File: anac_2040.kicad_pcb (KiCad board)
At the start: 2 copper layers, 53.2 x 68.2 mm, 62 parts, among them J1 Conn_01x02, J10 Debug, J5 Conn_01x09, J6 Barrel_Jack_MountingPin, J7 USB_C_Receptacle_USB2.0, Q1 PJA3432AU, Q2 PJA3432AU, SW1 SW_Push, SW2 SW_Push, U1 RP2040, U2 W25Q16JVSSIQ, U3 LM4040DBZ-3, U4 AP63203WU, Y1 Crystal_Small

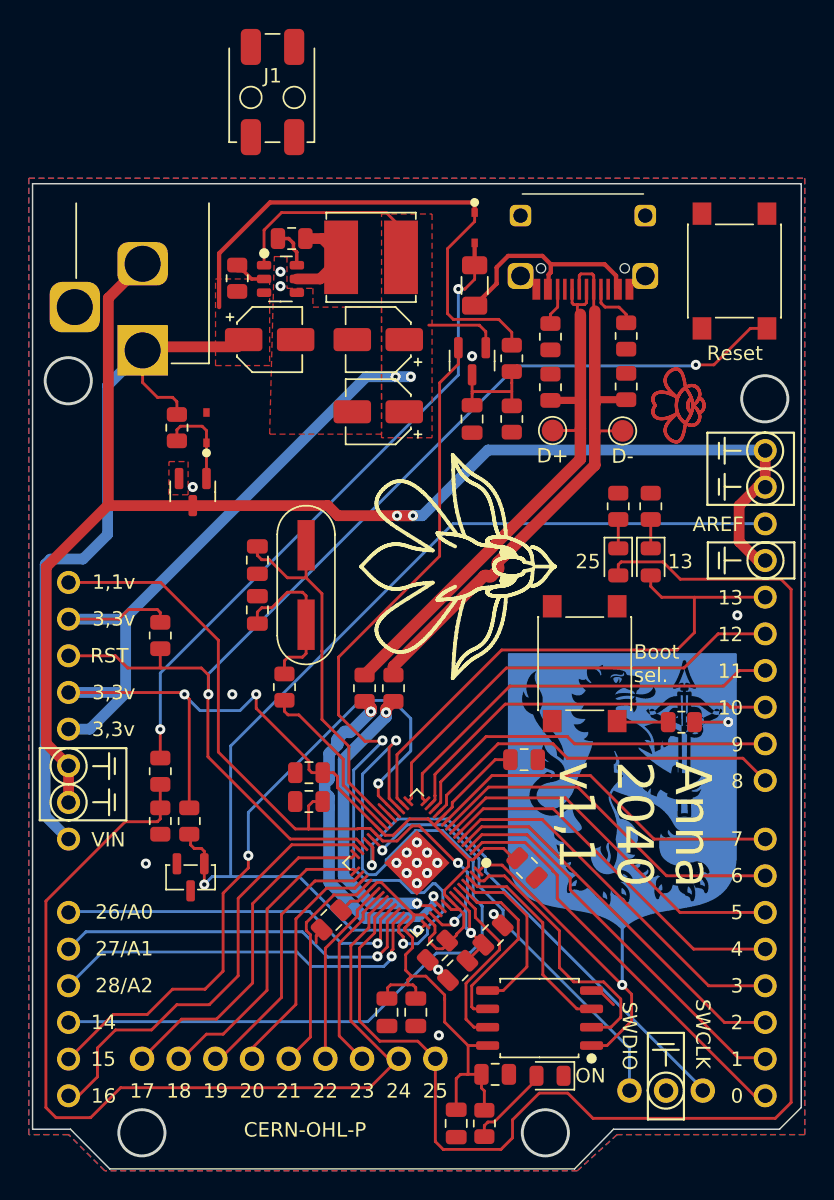
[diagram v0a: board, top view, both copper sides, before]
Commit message: small update
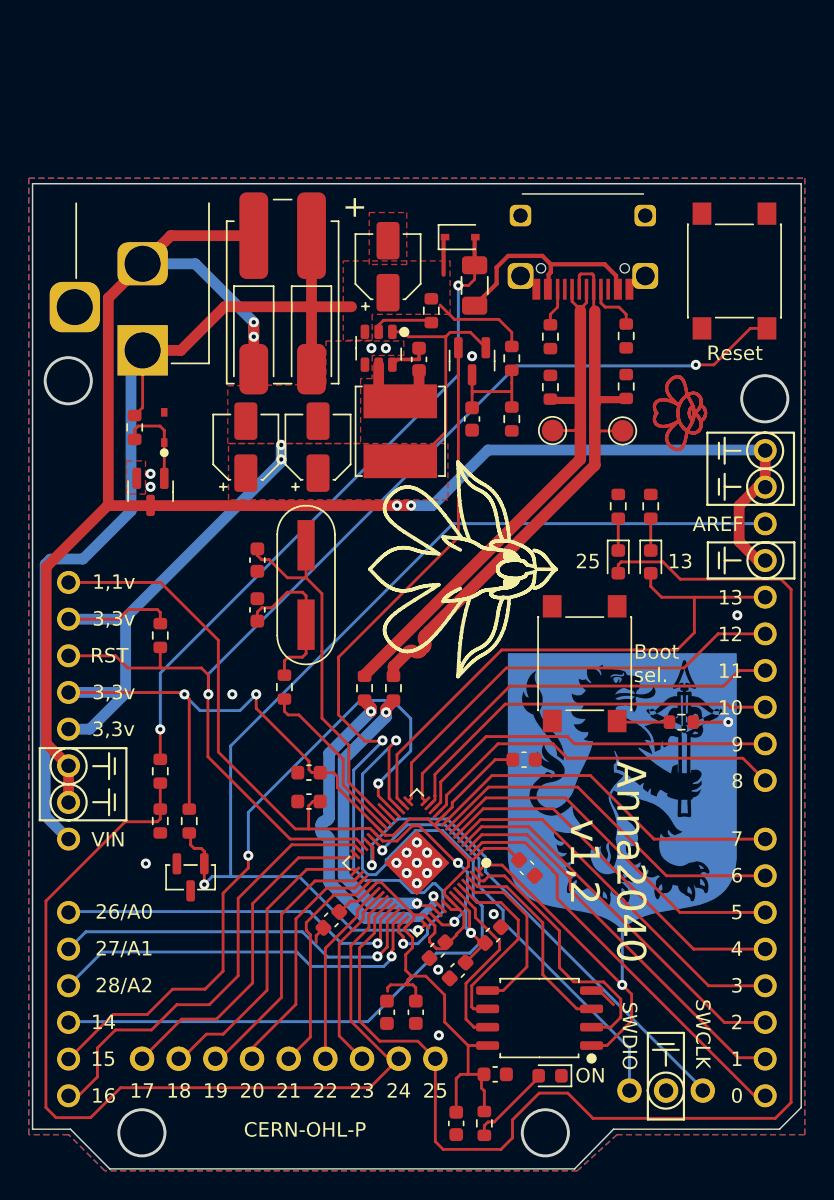
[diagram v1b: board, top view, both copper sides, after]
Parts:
- C1, C10, C11, C12, C13, C14, C15, C16, C2, C3, C4, C5, C6, C7, C8, C9: footprint Capacitor_SMD:C_0805_2012Metric -> Capacitor_SMD:C_0603_1608Metric
- D1: value D_Schottky -> D_Small
- D2, D3, D4: footprint LED_SMD:LED_0805_2012Metric -> LED_SMD:LED_0603_1608Metric
- J1: footprint DIY:WAGO terminal, 2P 3mm -> DIY:WAGO SMD terminal, 2P 4mm
- R1, R10, R11, R12, R13, R14, R15, R16, R17, R2, R3, R4, R5, R6, R7, R8, R9, RV1, RV2: footprint Resistor_SMD:R_0805_2012Metric -> Resistor_SMD:R_0603_1608Metric
- moved J1 13.8 mm to (145.7, 62.0)
- moved R9 13.6 mm to (156.0, 63.5), turned to -90 degrees
- moved L1 12.2 mm to (153.9, 71.8), turned to -90 degrees
- moved C16 12.2 mm to (155.2, 66.9), turned to -90 degrees
- moved C17 9.63 mm to (153.0, 60.5), turned to 90 degrees
- moved C18 9.50 mm to (143.2, 73.0), turned to 90 degrees
- moved C19 8.54 mm to (148.2, 73.0), turned to 90 degrees
- moved U4 8.32 mm to (152.4, 66.1), turned to -90 degrees
- moved D5 2.92 mm to (137.5, 71.6)
- moved R17 2.92 mm to (135.4, 71.6)
- moved Q2 2.92 mm to (136.6, 76.0)
- moved D1 1.19 mm to (158.0, 58.4), turned to 0 degrees
- renumbered D+ to TP1, D- to TP2
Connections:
- J1 pad 1: VSYS -> GND1
- J1 pad 2: GND1 -> VSYS
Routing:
- net GND1: track 98.0 -> 119.5 mm, vias 2 -> 4
- net +3.3V: track 172.6 -> 160.7 mm
- net VSYS: track 88.6 -> 77.6 mm
- net 3,3V_EN: track 2.10 -> 4.32 mm
- net VBUSPIN: track 45.1 -> 45.6 mm
- net GND: vias 19 -> 20
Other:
- board text added: "+"
- board text added: "Anna2040 v1,2"
- board text removed: "Anna 2040 v1,1"
